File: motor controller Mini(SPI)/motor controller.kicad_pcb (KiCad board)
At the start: 2 copper layers, 21 x 10.5 mm, 29 parts, among them IC1 MA702, IC2 ACS711KEXLT-15AB-T, IC3 MIC5501-3.0YM5-TR, IC4 A3918SESTR-T, J1 Conn_01x06_Male, J2 Conn_01x06_Male, J3 Conn_01x04_Male, M1 Motor_DC, U1 STM32L432KCUx, Y1 32mhz

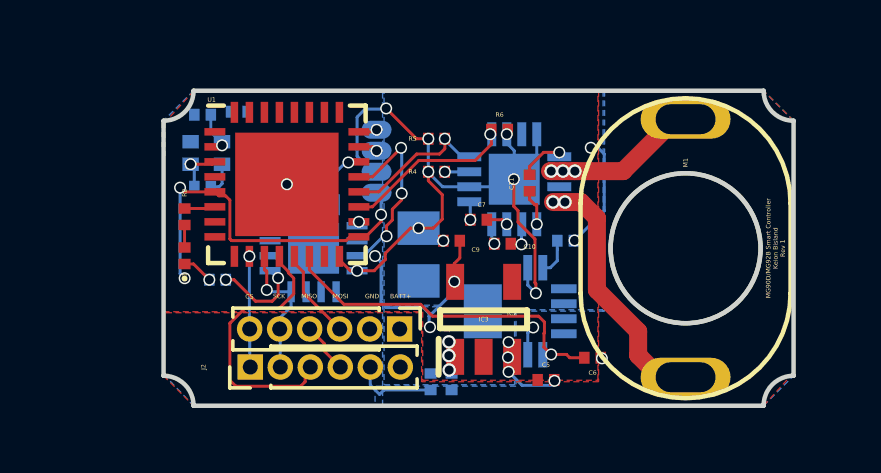
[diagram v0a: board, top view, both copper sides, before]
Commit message: Push to new server
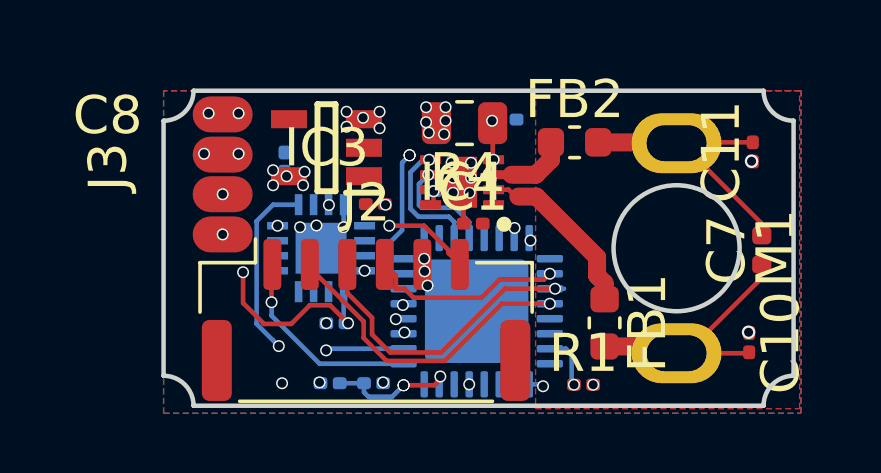
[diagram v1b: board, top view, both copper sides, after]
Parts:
- removed C12: 10Uf, Capacitor_SMD:C_0805_2012Metric
- removed C4, C5: 0.1Uf, Capacitor_SMD:C_0201_0603Metric
- removed D1: LED, LED_SMD:LED_0201_0603Metric
- removed IC2: ACS711KEXLT-15AB-T, ACS711KEXLT-15AB-T:EX-PACKAGE
- removed J1: Conn_01x06_Male, Connector_PinHeader_1.00mm:PinHeader_1x06_P1.00mm_Vertical
- removed R5, R6: 10K, Resistor_SMD:R_0201_0603Metric
- removed Y1: 32mhz, ECX-31B:ECX-1247
- added FB1: Ferrite_Bead, Inductor_SMD:L_0603_1608Metric, F.Cu at (14.7, 7.74)
- added FB2: Ferrite_Bead, Inductor_SMD:L_0603_1608Metric, F.Cu at (13.7, 1.72)
- C1: value 10pF -> 0.1uF; moved to F.Cu
- C10, C11: value 0.1Uf -> 100nF
- C2: value 10pF -> 0.1uF
- C3: value 1UF -> 1uF
- C6: value 0.1Uf -> 0.1UuF; moved to B.Cu
- C7: value 0.1Uf -> 47pF; footprint Capacitor_SMD:C_0201_0603Metric -> Capacitor_SMD:C_0402_1005Metric
- C8: value 1UF -> 1uF; moved to F.Cu
- C9: value 1UF -> 1uF; moved to B.Cu
- IC4: value A3918SESTR-T -> DRV8837CDSGT; footprint A3918SESTR-T:QFN50P300X300X80-17N-D -> DRV8837CDSGT:SON50P200X200X80-9N; moved to F.Cu
- J2: footprint Connector_PinHeader_1.00mm:PinHeader_1x06_P1.00mm_Vertical -> Connector_Molex:Molex_CLIK-Mate_502386-0670_1x06-1MP_P1.25mm_Horizontal
- J3, R1: moved to F.Cu
- M1: footprint hv5932mgMotor:hv5932mgMotor -> mg92b:mg92b
- R2: value 600 -> 1k; moved to B.Cu
- R3: value 10K -> 550
- R4: value 10K -> 0.33; footprint Resistor_SMD:R_0201_0603Metric -> Resistor_SMD:R_0805_2012Metric
- U1: moved to B.Cu
- moved R1 14.6 mm to (14.0, 9.80), turned to 0 degrees
- moved C1 9.72 mm to (10.3, 4.43), turned to 0 degrees
- moved C7 9.49 mm to (19.9, 5.31), turned to 90 degrees
- moved R3 9.18 mm to (5.55, 9.75)
- moved C10 8.86 mm to (19.5, 8.40), turned to 270 degrees
- moved C6 8.44 mm to (11.4, 0.96), turned to 180 degrees
- moved R2 8.40 mm to (7.00, 9.75), turned to 0 degrees
- moved C2 8.07 mm to (9.37, 3.34)
- moved IC3 7.76 mm to (5.43, 1.90), turned to 180 degrees
- moved U1 7.61 mm to (10.4, 7.35), turned to 90 degrees
- moved C11 7.51 mm to (19.6, 2.04)
- moved C8 6.44 mm to (7.06, 3.78), turned to 180 degrees
- moved C9 6.16 mm to (4.03, 2.38), turned to 90 degrees
- moved J3 5.15 mm to (1.97, 2.79), turned to 90 degrees
- moved C3 4.20 mm to (5.75, 7.75)
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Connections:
- C1 pad 1: Net-(C1-Pad1) -> GND
- C1 pad 2: GND -> +BATT
- C10 pad 1: Net-(C10-Pad1) -> GND
- C10 pad 2: Net-(C10-Pad2) -> OUT1
- C11 pad 1: Net-(C11-Pad1) -> GND
- C11 pad 2: MC+ -> OUT2
- C2 pad 2: Net-(C2-Pad2) -> +3V3
- C6 pad 1: FB -> GND
- C6 pad 2: GND -> FB
- C7 pad 1: Net-(C7-Pad1) -> OUT1
- C7 pad 2: Net-(C7-Pad2) -> OUT2
- IC1 pad 1: Net-(IC1-Pad1) -> (no net)
- IC1 pad 10: Net-(IC1-Pad10) -> (no net)
- IC1 pad 11: Net-(IC1-Pad11) -> (no net)
- IC1 pad 14: Net-(IC1-Pad14) -> (no net)
- IC1 pad 15: Net-(IC1-Pad15) -> (no net)
- IC1 pad 16: Net-(IC1-Pad16) -> (no net)
- IC1 pad 2: Net-(IC1-Pad2) -> (no net)
- IC1 pad 3: Net-(IC1-Pad3) -> (no net)
- IC1 pad 4: MOSI2 -> MOSI
- IC1 pad 6: Net-(IC1-Pad6) -> (no net)
- IC1 pad 7: MISO2 -> MISO
- IC1 pad 9: Net-(IC1-Pad9) -> (no net)
- IC3 pad 2: Net-(IC3-Pad2) -> (no net)
- IC3 pad 4: Net-(IC3-Pad4) -> (no net)
- IC4 pad 1: Net-(C7-Pad2) -> +BATT
- IC4 pad 2: GND -> Net-(FB1-Pad1)
- IC4 pad 3: Net-(IC4-Pad3) -> Net-(FB2-Pad1)
- IC4 pad 4: IN1 -> FB
- IC4 pad 6: GND -> IN1
- IC4 pad 7: Net-(IC4-Pad7) -> +3V3
- IC4 pad 8: GND -> +3V3
- IC4 pad 9: MC+ -> GND
- J2 pad 2: SCK -> MOSI2
- J2 pad 3: MISO -> MISO2
- J2 pad 4: Net-(J1-Pad4) -> SCK2
- R2 pad 1: Net-(D1-Pad2) -> PREF
- R2 pad 2: signaling -> +BATT
- R3 pad 1: Net-(IC2-Pad4) -> GND
- R3 pad 2: +3V3 -> PREF
- R4 pad 1: Net-(IC4-Pad3) -> FB
- U1 pad 10: CS -> ENC_CS
- U1 pad 14: FB -> (no net)
- U1 pad 15: Net-(U1-Pad15) -> FB
- U1 pad 18: ENC_CS -> (no net)
- U1 pad 2: Net-(C1-Pad1) -> (no net)
- U1 pad 21: MISO2 -> (no net)
- U1 pad 22: MOSI2 -> (no net)
- U1 pad 25: Net-(U1-Pad25) -> (no net)
- U1 pad 26: Net-(U1-Pad26) -> SCK2
- U1 pad 27: Net-(U1-Pad27) -> MISO2
- U1 pad 28: Net-(U1-Pad28) -> MOSI2
- U1 pad 29: Net-(U1-Pad29) -> (no net)
- U1 pad 3: Net-(C2-Pad2) -> (no net)
- U1 pad 30: Net-(U1-Pad30) -> (no net)
- U1 pad 4: Net-(U1-Pad4) -> (no net)
- U1 pad 6: signaling -> (no net)
- U1 pad 7: Net-(U1-Pad7) -> PREF
- U1 pad 8: Net-(U1-Pad8) -> (no net)
- U1 pad 9: Net-(U1-Pad9) -> CS
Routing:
- net GND: track 33.0 -> 6.32 mm, vias 16 -> 31
- net +3V3: track 27.3 -> 15.3 mm, vias 11 -> 13
- net ENC_CS: track 0.15 -> 10.3 mm, vias 1 -> 2
- net SWDIO: track 0.64 -> 10.5 mm, vias 1 -> 2
- net SWCLK: track 0.62 -> 10.4 mm, vias 1 -> 2
- net +BATT: track 0.00 -> 9.30 mm, vias 3 -> 2
- net MOSI2: track 1.99 -> 10.5 mm
- net SCK2: track 0.00 -> 6.58 mm, vias 0 -> 1
- net Net-(FB1-Pad1): track 0.00 -> 6.49 mm
- net MOSI: track 3.05 -> 9.12 mm, vias 0 -> 2
- net MISO: track 9.10 -> 4.73 mm, vias 0 -> 2
- net OUT2: track 5.24 -> 9.54 mm, vias 3 -> 0
- net MISO2: track 6.23 -> 10.4 mm, vias 3 -> 1
- net PREF: track 0.00 -> 4.03 mm, vias 0 -> 3
- net Net-(FB2-Pad1): track 0.00 -> 3.42 mm
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- added copper zone on In1.Cu, net +3V3
- added copper zone on F.Cu, net +BATT
- added copper zone on In2.Cu, net GND
- removed copper zone on F.Cu, net +3V3
- removed copper zone on B.Cu, net +BATT
- removed copper zone on B.Cu, net MC+
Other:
- outline, holes or cut-outs redrawn
- copper layers 2 -> 4
- net class Default: clearance 0.1 -> 0.127; trace_width 0.1 -> 0.154
- net class Power: clearance 0.1 -> 0.127
- rule trace_clearance: 0.1 -> 0.127
- rule trace_min: 0.1 -> 0.127
- board text removed: "BATT+"
- board text removed: "CS"
- board text removed: "GND"
- board text removed: "MG90D/MG92B Smart Controller Keion Bisland Rev 1"
- board text removed: "MISO"
- board text removed: "MOSI"
- board text removed: "SCK"
